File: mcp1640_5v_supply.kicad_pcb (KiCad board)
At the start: 2 copper layers, 16.8 x 9.7 mm, 8 parts, among them J1 Conn_01x03, U1 MCP1640CH

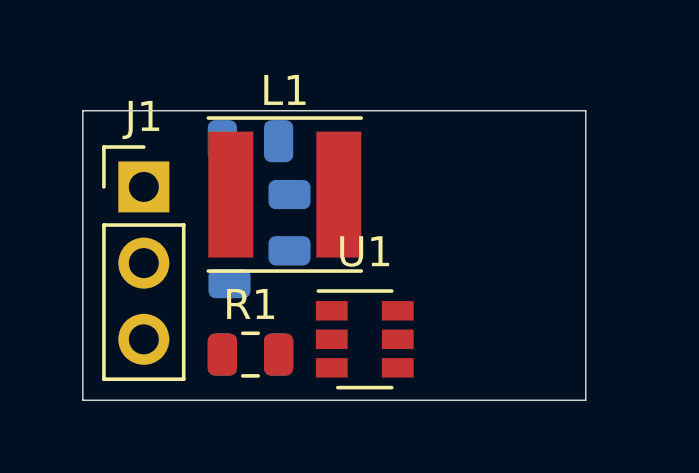
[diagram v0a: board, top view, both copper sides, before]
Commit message: Finished module (probably)
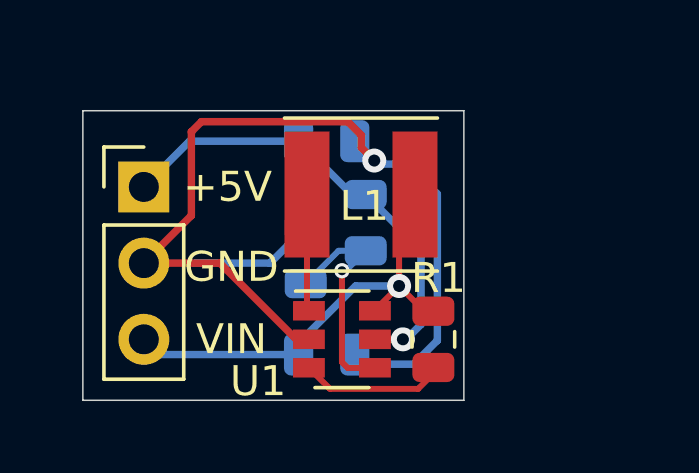
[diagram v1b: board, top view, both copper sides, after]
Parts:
- moved R1 6.12 mm to (145.8, 101.1), turned to 270 degrees
- moved C1 2.54 mm to (142.2, 101.6)
- moved C2 2.54 mm to (142.2, 94.5)
- moved L1 2.54 mm to (143.4, 96.3), turned to 180 degrees
- moved R2 2.54 mm to (143.5, 97.2)
- moved R3 2.54 mm to (141.5, 98.3)
- moved U1 0.76 mm to (142.7, 101.1)
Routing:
- net GND: track 0.00 -> 36.6 mm, vias 0 -> 1
- net VIN: track 0.00 -> 16.3 mm, vias 0 -> 1
- net +5V: track 0.00 -> 15.6 mm, vias 0 -> 1
- net Net-(R2-Pad2): track 0.00 -> 7.75 mm, vias 0 -> 1
- net Net-(R1-Pad2): track 0.00 -> 4.85 mm
- net Net-(L1-Pad2): track 0.00 -> 3.90 mm
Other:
- board size 16.8 x 9.7 mm -> 12.7 x 9.7 mm
- board text added: "+5V"
- board text added: "GND"
- board text added: "VIN"
- board text added: "WM v0.0.0 04/09/20"

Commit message: Another revision
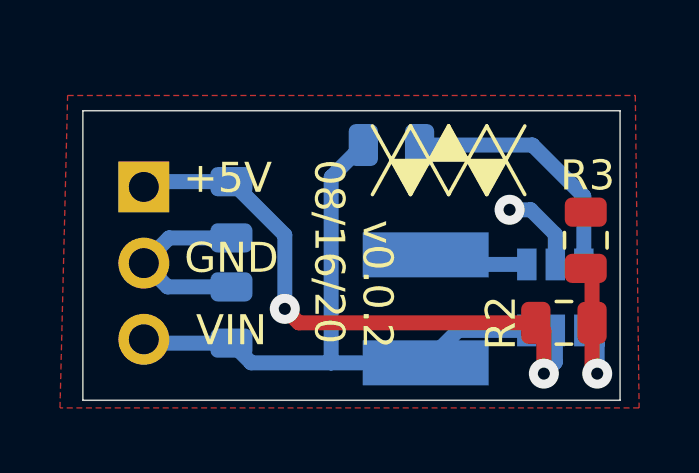
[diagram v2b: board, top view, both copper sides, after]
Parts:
- added REF**: Logo_WM, Symbol:Logo_WM, F.Cu at (146.3, 95.1)
- J1, L1, R1, U1: moved to B.Cu
- R2, R3: moved to F.Cu
- moved R3 9.35 mm to (150.9, 97.8)
- moved R2 7.40 mm to (150.1, 100.5), turned to 0 degrees
- moved U1 7.25 mm to (149.9, 99.7), turned to 270 degrees
- moved R1 6.63 mm to (144.4, 94.6), turned to 0 degrees
- moved L1 4.38 mm to (145.5, 100.1), turned to 90 degrees
- moved C2 3.91 mm to (139.1, 96.8), turned to 270 degrees
- moved C1 3.44 mm to (139.1, 100.3), turned to 90 degrees
- turned J1 to 180 degrees
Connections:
- net Net-(R2-Pad2) renamed FBACK
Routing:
- net GND: track 36.6 -> 9.38 mm
- net +5V: track 15.6 -> 19.9 mm, vias 1 -> 2
- net VIN: track 16.3 -> 20.1 mm, vias 1 -> 0
- net Net-(R1-Pad2): track 4.85 -> 8.45 mm
- net FBACK: track 7.75 -> 5.39 mm
- added copper zone on F.Cu, net GND
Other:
- board size 12.7 x 9.7 mm -> 17.9 x 9.7 mm
- board text added: "v0.0.2 08/16/20"
- board text removed: "WM v0.0.0 04/09/20"
